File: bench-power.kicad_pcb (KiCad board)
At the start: 2 copper layers, 34 parts, among them J1 16PIN

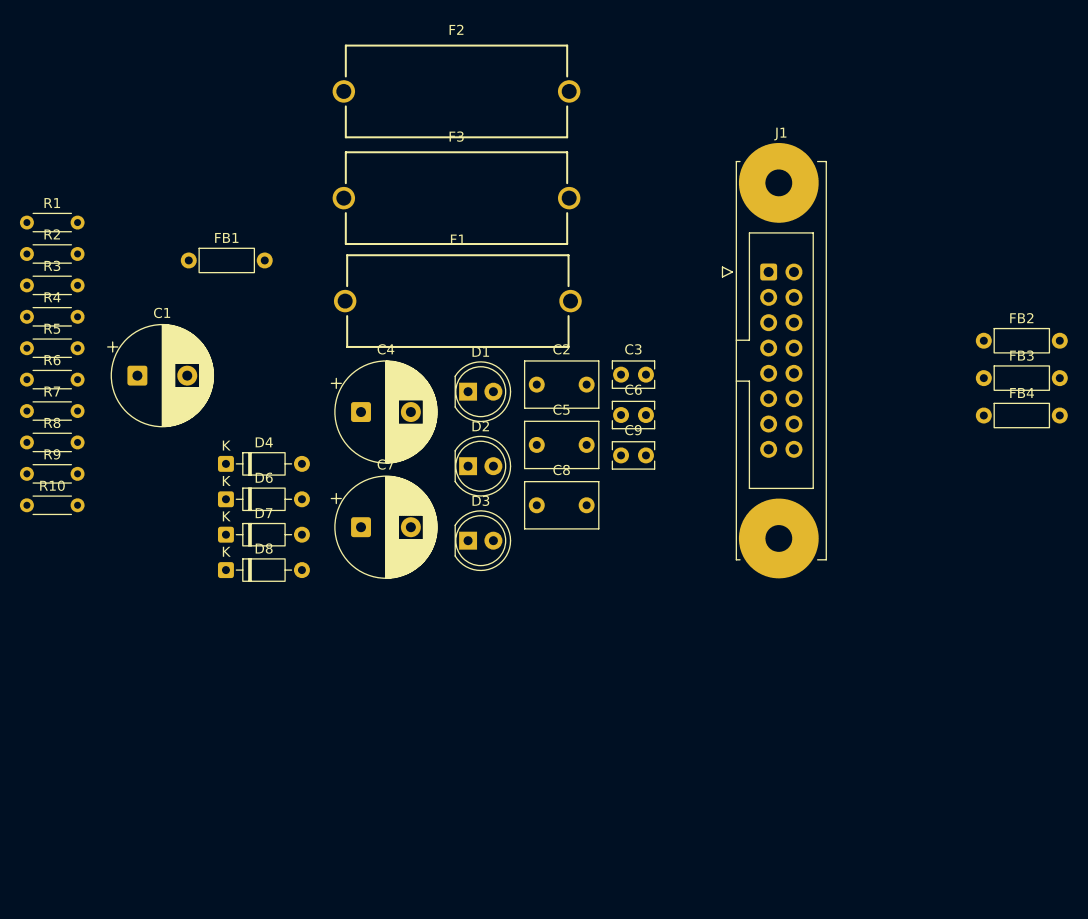
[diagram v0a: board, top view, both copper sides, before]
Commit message: prototype candidate
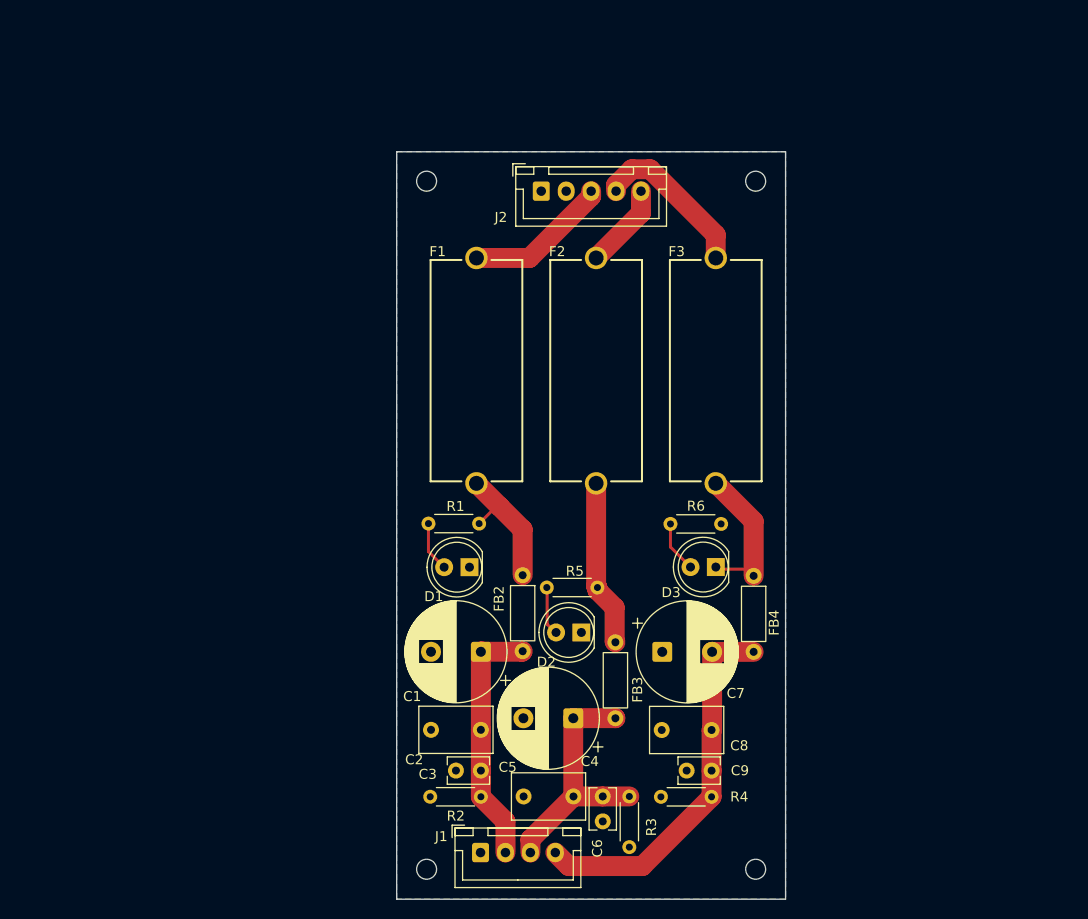
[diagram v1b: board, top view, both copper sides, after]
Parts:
- removed D4, D6, D7, D8: 1N4148, Diode_THT:D_DO-35_SOD27_P7.62mm_Horizontal
- removed FB1: 100@100MHz, Inductor_THT:L_Axial_L5.3mm_D2.2mm_P7.62mm_Horizontal_Vishay_IM-1
- removed R10, R9: 100k, Resistor_THT:R_Axial_DIN0204_L3.6mm_D1.6mm_P5.08mm_Horizontal
- removed R7, R8: 4.7k, Resistor_THT:R_Axial_DIN0204_L3.6mm_D1.6mm_P5.08mm_Horizontal
- added J2: POWER_IN_BRD, Connector_JST:JST_XH_B5B-XH-A_1x05_P2.50mm_Vertical, F.Cu at (154.5, 52.0)
- added REF**: MountingHole_2mm, MountingHole:MountingHole_2mm, F.Cu at (143.0, 120.0)
- added REF**: MountingHole_2mm, MountingHole:MountingHole_2mm, F.Cu at (176.0, 51.0)
- added REF**: MountingHole_2mm, MountingHole:MountingHole_2mm, F.Cu at (176.0, 120.0)
- added REF**: MountingHole_2mm, MountingHole:MountingHole_2mm, F.Cu at (143.0, 51.0)
- J1: value 16PIN -> PWR_OUT; footprint Connector_IDC:IDC-Header_2x08-1MP_P2.54mm_Latch_Vertical -> Connector_JST:JST_XH_B4B-XH-A_1x04_P2.50mm_Vertical
- moved R3 82.6 mm to (163.3, 117.8), turned to 90 degrees
- moved R4 79.7 mm to (166.5, 112.7)
- moved R2 67.8 mm to (143.4, 112.7)
- moved R6 66.1 mm to (167.5, 85.4)
- moved J1 65.0 mm to (148.4, 118.3)
- moved R5 62.0 mm to (160.1, 91.7), turned to 180 degrees
- moved R1 54.5 mm to (148.3, 85.3), turned to 180 degrees
- moved FB2 51.9 mm to (152.6, 90.5), turned to -90 degrees
- moved FB3 45.5 mm to (161.9, 97.2), turned to -90 degrees
- moved C1 44.2 mm to (148.4, 98.2), turned to 180 degrees
- moved C3 43.0 mm to (145.9, 110.1)
- moved C6 40.8 mm to (160.7, 115.2), turned to 90 degrees
- moved C4 37.4 mm to (157.7, 104.9), turned to 180 degrees
- moved C2 36.2 mm to (143.4, 106.0)
- moved C5 35.3 mm to (152.7, 112.7)
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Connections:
- C1 pad 1: Net-(J1-Pin_11) -> Net-(J1-Pin_2)
- C1 pad 2: Earth -> GND
- C2 pad 1: Earth -> GND
- C2 pad 2: Net-(J1-Pin_11) -> Net-(J1-Pin_2)
- C3 pad 1: Earth -> GND
- C3 pad 2: Net-(J1-Pin_11) -> Net-(J1-Pin_2)
- C4 pad 1: Net-(J1-Pin_10) -> Net-(J1-Pin_3)
- C4 pad 2: Earth -> GND
- C5 pad 1: Earth -> GND
- C5 pad 2: Net-(J1-Pin_10) -> Net-(J1-Pin_3)
- C6 pad 1: Earth -> GND
- C6 pad 2: Net-(J1-Pin_10) -> Net-(J1-Pin_3)
- C7 pad 1: Earth -> GND
- C7 pad 2: Net-(J1-Pin_1) -> Net-(J1-Pin_4)
- C8 pad 1: Earth -> GND
- C8 pad 2: Net-(J1-Pin_1) -> Net-(J1-Pin_4)
- C9 pad 1: Earth -> GND
- C9 pad 2: Net-(J1-Pin_1) -> Net-(J1-Pin_4)
- D1 pad 1: Earth -> GND
- D2 pad 1: Earth -> GND
- F1 pad 1: Net-(F1-Pad1) -> /+5Vout
- F2 pad 1: Net-(F2-Pad1) -> /+Vout
- FB2 pad 2: Net-(J1-Pin_11) -> Net-(J1-Pin_2)
- FB3 pad 2: Net-(J1-Pin_10) -> Net-(J1-Pin_3)
- FB4 pad 2: Net-(J1-Pin_1) -> Net-(J1-Pin_4)
- J1 pad 1: Net-(J1-Pin_1) -> GND
- J1 pad 2: Net-(J1-Pin_1) -> Net-(J1-Pin_2)
- J1 pad 3: Earth -> Net-(J1-Pin_3)
- J1 pad 4: Earth -> Net-(J1-Pin_4)
- R2 pad 1: Earth -> GND
- R2 pad 2: Net-(J1-Pin_11) -> Net-(J1-Pin_2)
- R3 pad 1: Earth -> GND
- R3 pad 2: Net-(J1-Pin_10) -> Net-(J1-Pin_3)
- R4 pad 1: Earth -> GND
- R4 pad 2: Net-(J1-Pin_1) -> Net-(J1-Pin_4)
- R6 pad 2: Earth -> GND
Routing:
- net Net-(J1-Pin_4): track 0.00 -> 37.8 mm
- net Net-(J1-Pin_2): track 0.00 -> 25.5 mm
- net Net-(J1-Pin_3): track 0.00 -> 25.1 mm
- net +12V: track 0.00 -> 16.7 mm
- net /-Vout: track 0.00 -> 16.3 mm
- net -12V: track 0.00 -> 15.0 mm
- net /+5Vout: track 0.00 -> 14.9 mm
- net +5V: track 0.00 -> 13.9 mm
- net /+Vout: track 0.00 -> 8.56 mm
- net Net-(D3-A): track 0.00 -> 5.18 mm
- net Net-(D1-A): track 0.00 -> 5.02 mm
- net Net-(D2-A): track 0.00 -> 4.93 mm
- added copper zone on B.Cu, net GND
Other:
- board outline added: 39 x 75 mm
